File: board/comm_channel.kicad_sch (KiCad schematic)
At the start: 25 parts, among them J401 JST_B13P_XH, U401 EL357N(C)(TA)-G, U402 EL357N(C)(TA)-G, U403 EL357N(C)(TA)-G, U404 EL357N(C)(TA)-G, U405 EL357N(C)(TA)-G

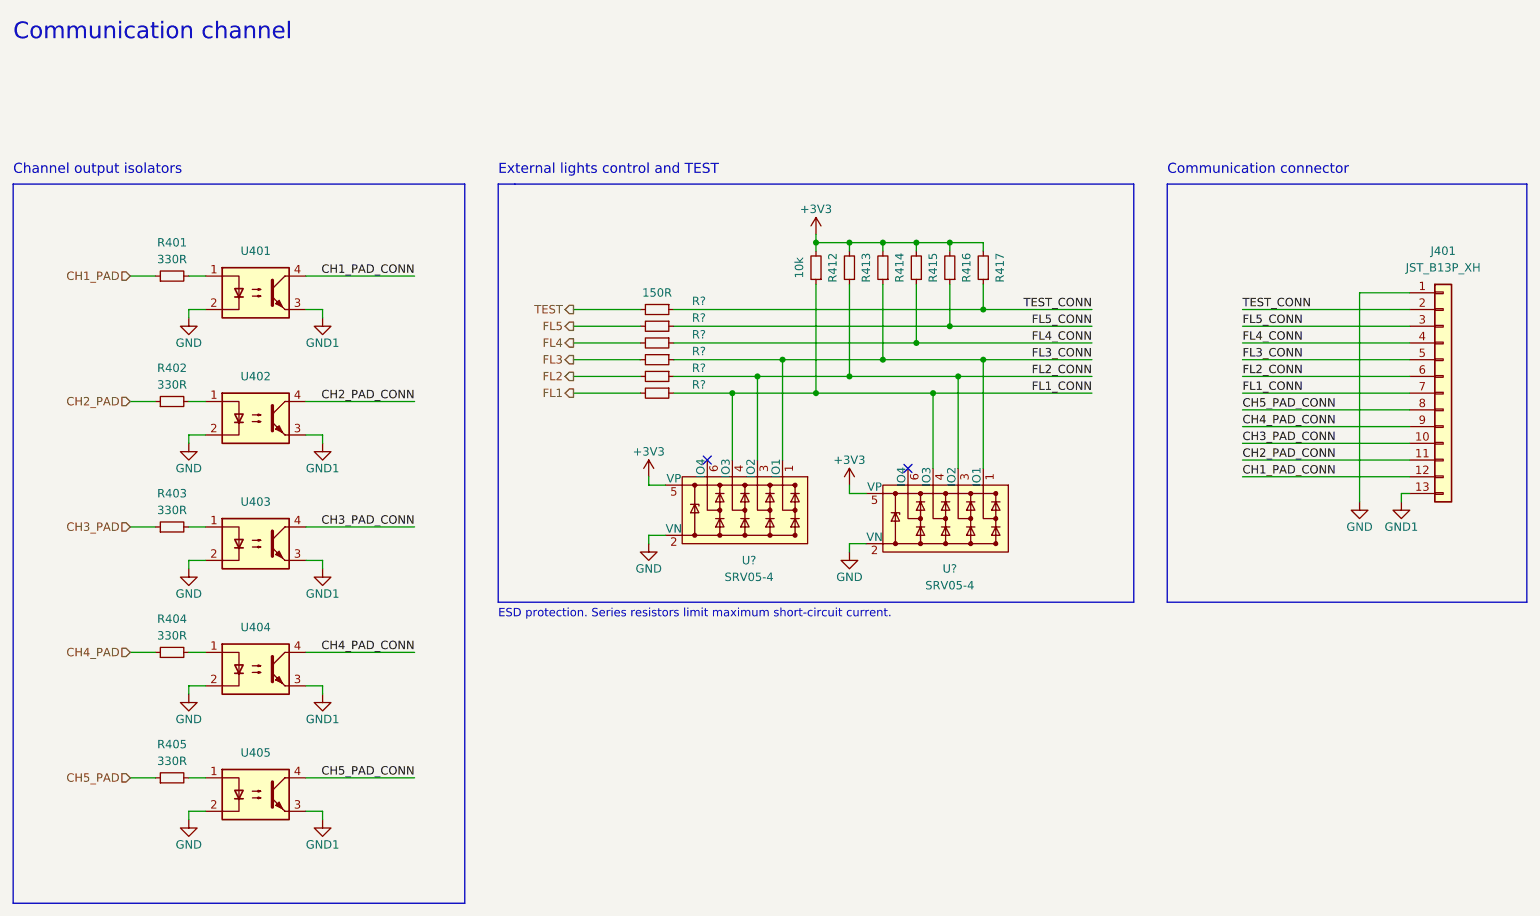
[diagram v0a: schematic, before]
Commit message: Update PCB
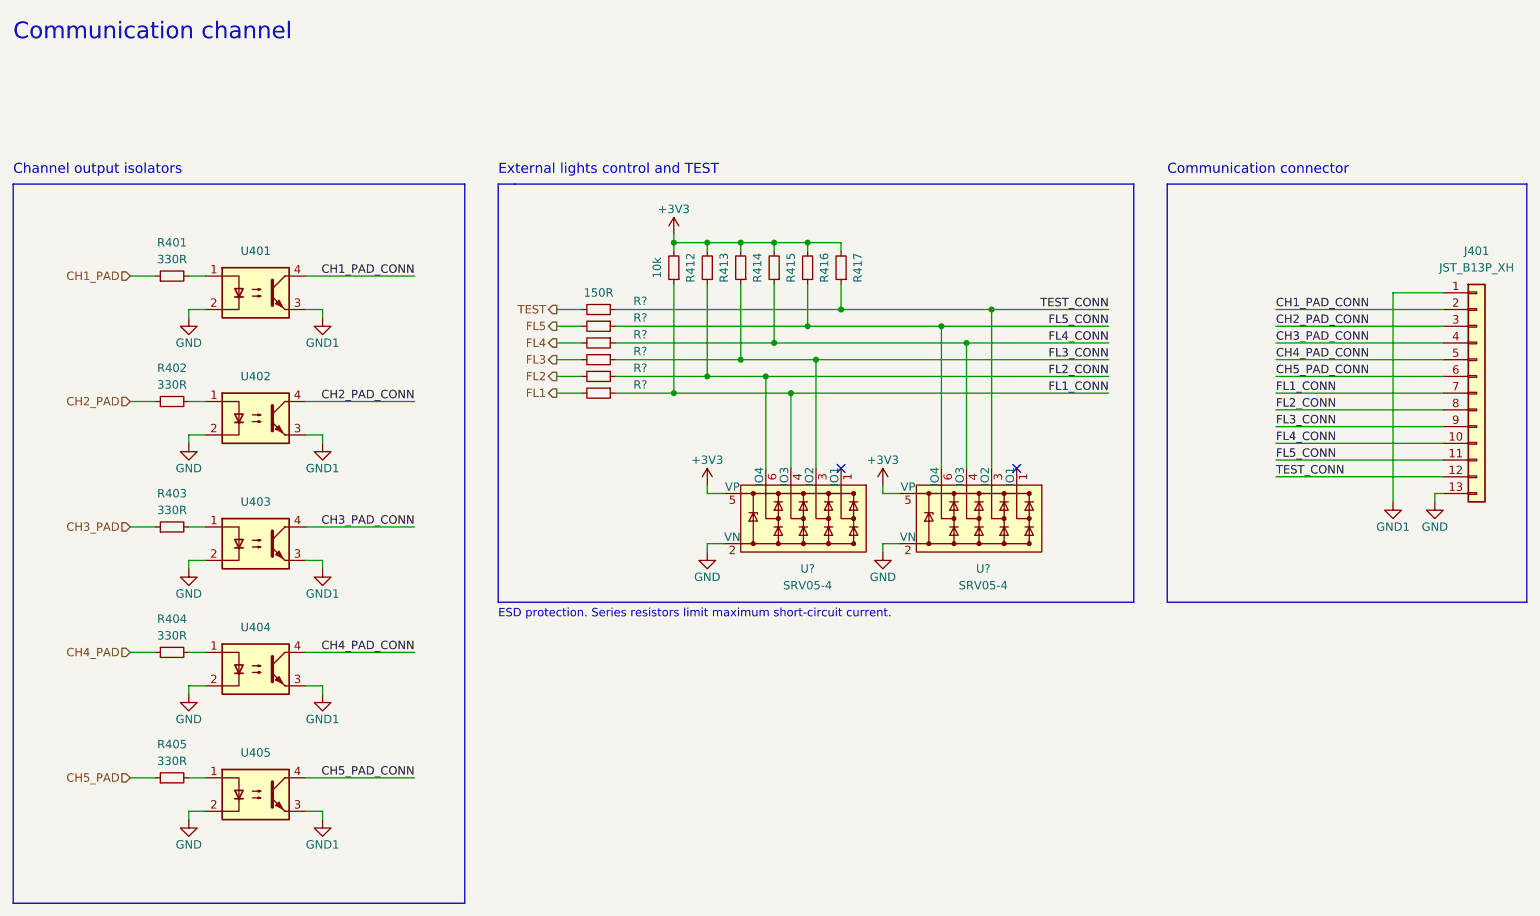
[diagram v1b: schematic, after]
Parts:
- J401: footprint Connector_JST:JST_XH_B13B-XH-A_1x13_P2.50mm_Vertical -> ProjectLibrary:JST_NH_B13P-SHF-1AA_1x13_P2.50mm_Vertical
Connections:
- net CH1_PAD_CONN: now also J401.2 (Pin_2); no longer J401.12 (Pin_12)
- net CH2_PAD_CONN: now also J401.3 (Pin_3); no longer J401.11 (Pin_11)
- net CH3_PAD_CONN: now also J401.4 (Pin_4); no longer J401.10 (Pin_10)
- net CH4_PAD_CONN: now also J401.5 (Pin_5); no longer J401.9 (Pin_9)
- net CH5_PAD_CONN: now also J401.6 (Pin_6); no longer J401.8 (Pin_8)
- net FL1_CONN: no longer U?.4 (IO3)
- net FL2_CONN: now also J401.8 (Pin_8), U?.6 (IO4); no longer J401.6 (Pin_6), U?.3 (IO2), U?.3 (IO2)
- net FL3_CONN: now also J401.9 (Pin_9), U?.3 (IO2); no longer J401.5 (Pin_5), U?.1 (IO1), U?.1 (IO1)
- net FL4_CONN: now also J401.10 (Pin_10), U?.4 (IO3); no longer J401.4 (Pin_4)
- net FL5_CONN: now also J401.11 (Pin_11), U?.6 (IO4); no longer J401.3 (Pin_3)
- net GND: now also J401.13 (Pin_13); no longer J401.1 (Pin_1)
- net GND1: now also J401.1 (Pin_1); no longer J401.13 (Pin_13)
- net TEST_CONN: now also J401.12 (Pin_12), U?.3 (IO2); no longer J401.2 (Pin_2)
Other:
- moved on the sheet: R412, R413, R414, R415, R416, R417, R?, U?
